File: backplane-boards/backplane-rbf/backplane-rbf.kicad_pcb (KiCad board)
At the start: 2 copper layers, 43 x 10 mm, 3 parts, among them J1 Breakout Connector, J2 Breakout Connector

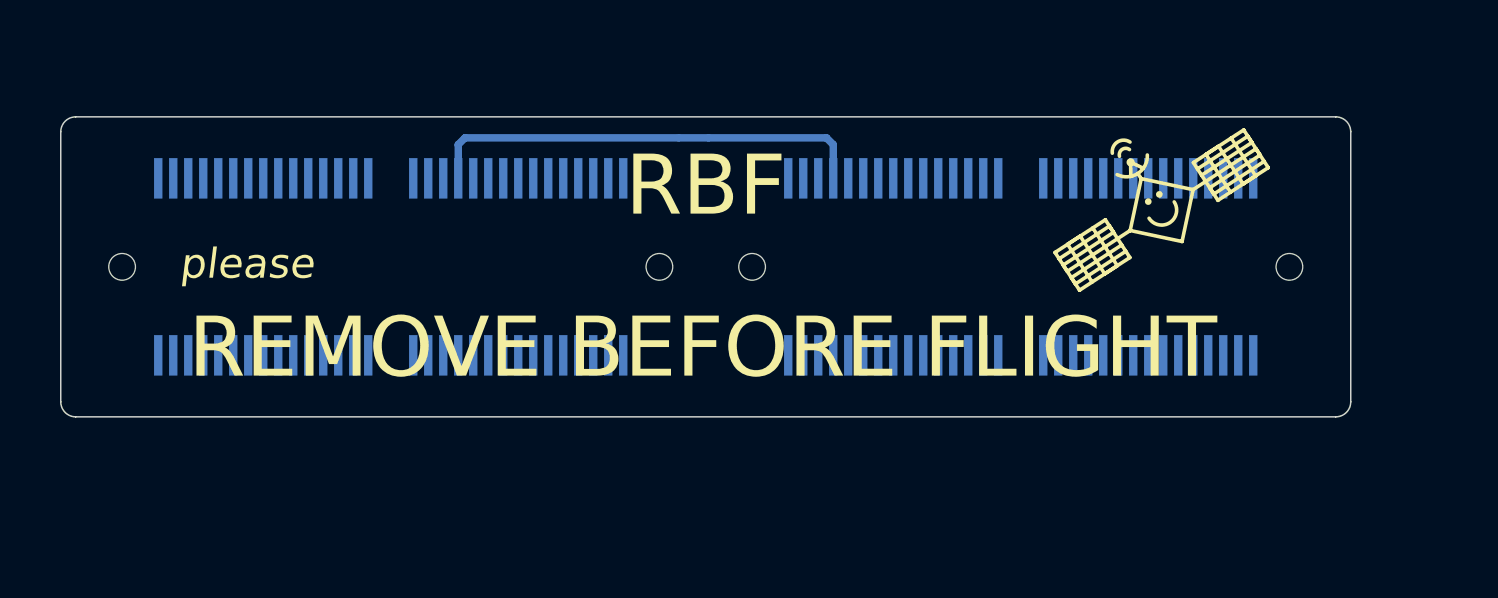
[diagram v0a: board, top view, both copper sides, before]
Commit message: rbf
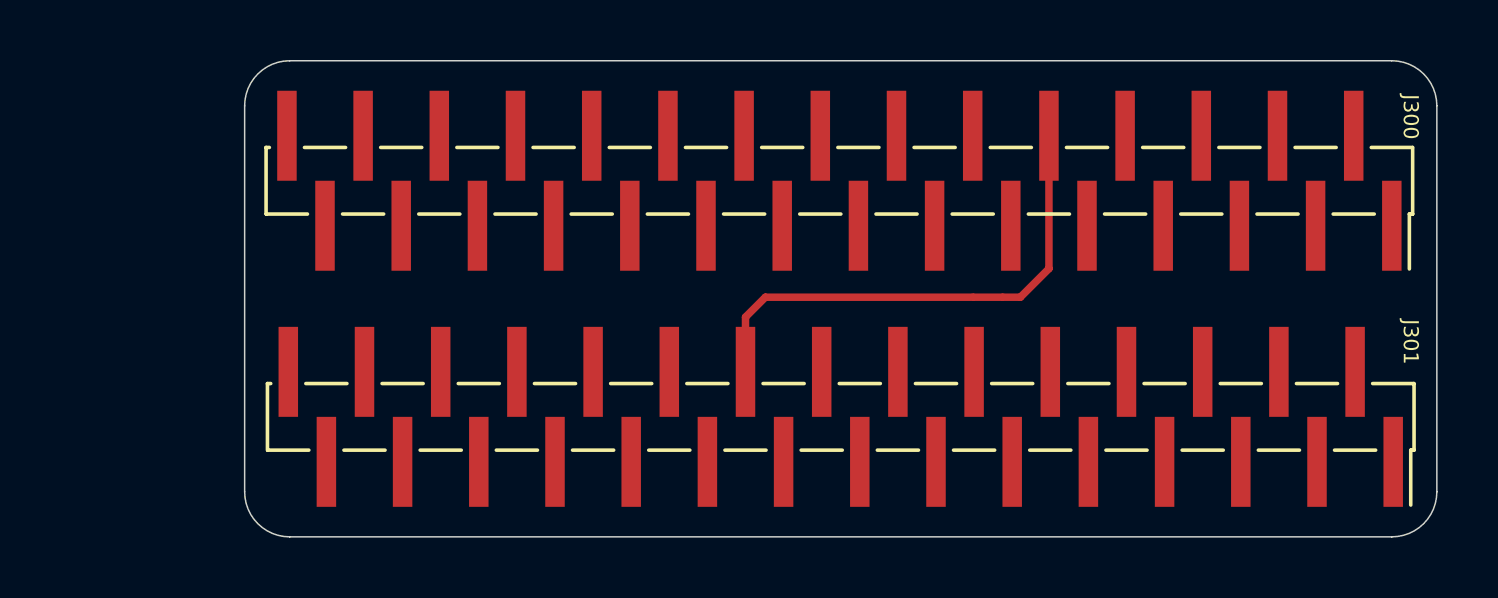
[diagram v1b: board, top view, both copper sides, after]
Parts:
- removed J1, J2: Breakout Connector, backplane-rbf:SAMTEC_LSH-030-01-X-D-A-TR
- added J300: FTS-130-01-L-SV, backplane-rbf:FTS-130-01-L-SV, F.Cu at (140.0, 92.1)
- added J301: FTS-130-01-L-SV, backplane-rbf:FTS-130-01-L-SV, F.Cu at (140.0, 100.0)
- NT1: moved to F.Cu
- moved NT1 11.2 mm to (144.9, 96.0), turned to 180 degrees
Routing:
- net /GND: track 5.37 -> 9.68 mm
- net /RBF: track 8.57 -> 6.36 mm
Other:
- board size 43 x 10 mm -> 39.7 x 15.9 mm
